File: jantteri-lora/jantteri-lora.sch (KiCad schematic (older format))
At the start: 0 parts

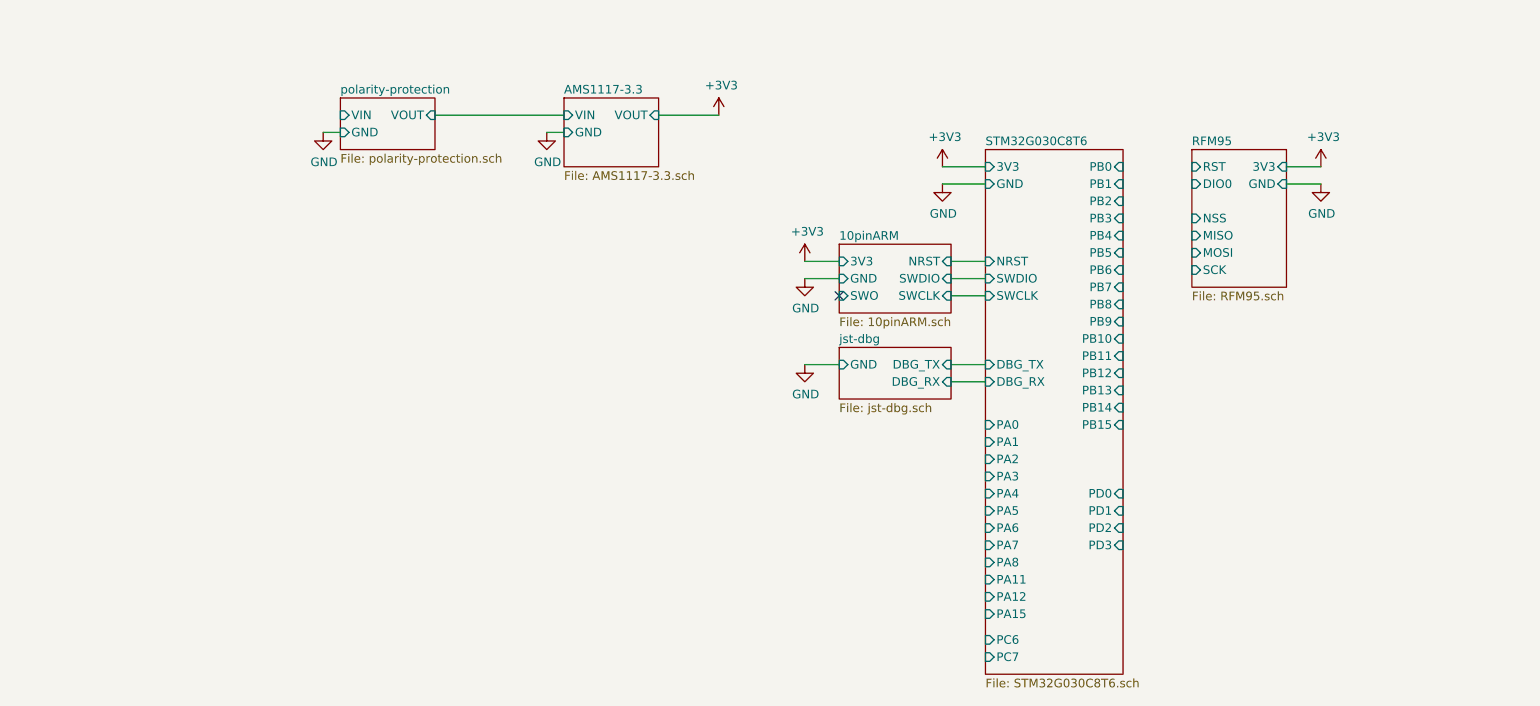
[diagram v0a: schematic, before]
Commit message: Lora PCB desging
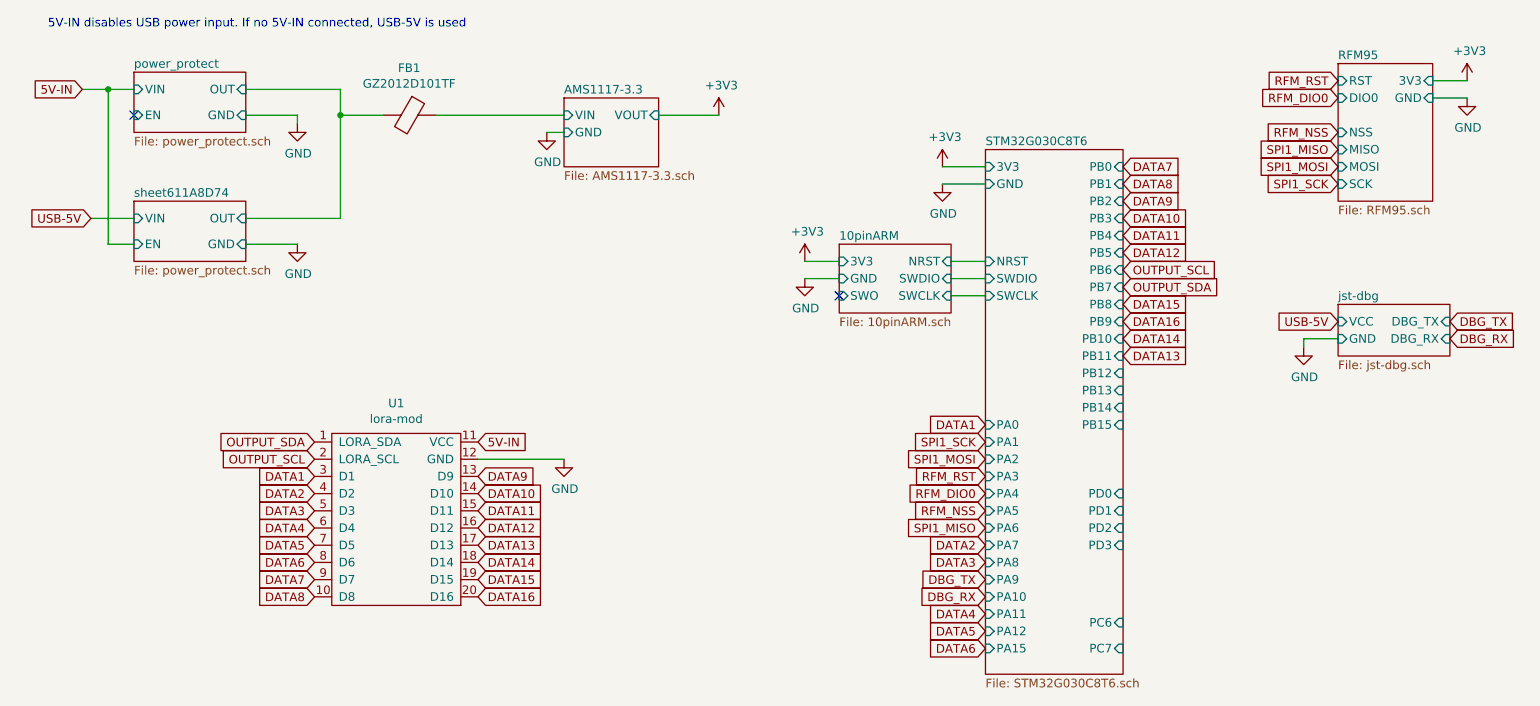
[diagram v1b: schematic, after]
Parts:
- added FB1: GZ2012D101TF, Inductor_SMD:L_0805_2012Metric, symbol Device:Ferrite_Bead
- added U1: lora-mod, RF_Module:HOPERF_RFM69HW, symbol voja-lib:lora-mod
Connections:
- net AMS1117-3.3/VIN: now also FB1.1
- net GND: now also U1.12 (GND)
- new net 5V-IN: U1.11 (VCC)
- new net DATA1: U1.3 (D1)
- new net DATA10: U1.14 (D10)
- new net DATA11: U1.15 (D11)
- new net DATA12: U1.16 (D12)
- new net DATA13: U1.17 (D13)
- new net DATA14: U1.18 (D14)
- new net DATA15: U1.19 (D15)
- new net DATA16: U1.20 (D16)
- new net DATA2: U1.4 (D2)
- new net DATA3: U1.5 (D3)
- new net DATA4: U1.6 (D4)
- new net DATA5: U1.7 (D5)
- new net DATA6: U1.8 (D6)
- new net DATA7: U1.9 (D7)
- new net DATA8: U1.10 (D8)
- new net DATA9: U1.13 (D9)
- new net OUTPUT_SCL: U1.2 (LORA_SCL)
- new net OUTPUT_SDA: U1.1 (LORA_SDA)
- new net power_protect/OUT: FB1.2
- no-connect marks 1 -> 2
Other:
- note added: "5V-IN disables USB power input. If no 5V-IN connected, USB-5V is used"

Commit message: Lora-module v1
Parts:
- U1: footprint RF_Module:HOPERF_RFM69HW -> voja-footprints:lora-mod; symbol voja-lib:lora-mod -> jantteri-lora-rescue:lora-mod-voja-lib
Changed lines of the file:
@@
 $EndSheet
 $Comp
-L power:+3V3 #PWR0101
+L power:+3V3 #PWR08
 U 1 1 61143103
 P 5850 1850
-F 0 "#PWR0101" H 5850 1700 50  0001 C CNN
+F 0 "#PWR08" H 5850 1700 50  0001 C CNN
 F 1 "+3V3" H 5865 2023 50  0000 C CNN
 F 2 "" H 5850 1850 50  0001 C CNN
@@
 $EndComp
 $Comp
-L power:GND #PWR0102
+L power:GND #PWR09
 U 1 1 611435CD
 P 5850 1950
-F 0 "#PWR0102" H 5850 1700 50  0001 C CNN
+F 0 "#PWR09" H 5850 1700 50  0001 C CNN
 F 1 "GND" H 5855 1777 50  0000 C CNN
 F 2 "" H 5850 1950 50  0001 C CNN
@@
 	6100 2600 5900 2600
 $Comp
-L power:GND #PWR0103
+L power:GND #PWR07
 U 1 1 611483EC
 P 5050 2500
-F 0 "#PWR0103" H 5050 2250 50  0001 C CNN
+F 0 "#PWR07" H 5050 2250 50  0001 C CNN
 F 1 "GND" H 5055 2327 50  0000 C CNN
 F 2 "" H 5050 2500 50  0001 C CNN
@@
 $EndComp
 $Comp
-L power:GND #PWR0104
+L power:GND #PWR010
 U 1 1 61148B21
 P 7950 2900
-F 0 "#PWR0104" H 7950 2650 50  0001 C CNN
+F 0 "#PWR010" H 7950 2650 50  0001 C CNN
 F 1 "GND" H 7955 2727 50  0000 C CNN
 F 2 "" H 7950 2900 50  0001 C CNN
@@
 $EndComp
 $Comp
-L power:+3V3 #PWR0105
+L power:+3V3 #PWR06
 U 1 1 61148EAA
 P 5050 2400
-F 0 "#PWR0105" H 5050 2250 50  0001 C CNN
+F 0 "#PWR06" H 5050 2250 50  0001 C CNN
 F 1 "+3V3" H 5065 2573 50  0000 C CNN
 F 2 "" H 5050 2400 50  0001 C CNN
@@
 	5250 2400 5050 2400
 $Comp
-L power:+3V3 #PWR0106
+L power:+3V3 #PWR011
 U 1 1 6114B431
 P 8900 1350
-F 0 "#PWR0106" H 8900 1200 50  0001 C CNN
+F 0 "#PWR011" H 8900 1200 50  0001 C CNN
 F 1 "+3V3" H 8915 1523 50  0000 C CNN
 F 2 "" H 8900 1350 50  0001 C CNN
@@
 $EndComp
 $Comp
-L power:GND #PWR0107
+L power:GND #PWR012
 U 1 1 6114B78E
 P 8900 1450
-F 0 "#PWR0107" H 8900 1200 50  0001 C CNN
+F 0 "#PWR012" H 8900 1200 50  0001 C CNN
 F 1 "GND" H 8905 1277 50  0000 C CNN
 F 2 "" H 8900 1450 50  0001 C CNN
@@
 	8700 1350 8900 1350
 $Comp
-L power:GND #PWR0108
+L power:GND #PWR03
 U 1 1 6114C811
 P 3550 1650
-F 0 "#PWR0108" H 3550 1400 50  0001 C CNN
+F 0 "#PWR03" H 3550 1400 50  0001 C CNN
 F 1 "GND" H 3555 1477 50  0000 C CNN
 F 2 "" H 3550 1650 50  0001 C CNN
@@
 	3550 1650 3650 1650
 $Comp
-L power:+3V3 #PWR0110
+L power:+3V3 #PWR05
 U 1 1 6114D52E
 P 4550 1550
-F 0 "#PWR0110" H 4550 1400 50  0001 C CNN
+F 0 "#PWR05" H 4550 1400 50  0001 C CNN
 F 1 "+3V3" H 4565 1723 50  0000 C CNN
 F 2 "" H 4550 1550 50  0001 C CNN
@@
 5V-IN
 $Comp
-L power:GND #PWR0109
+L power:GND #PWR04
 U 1 1 61169965
 P 3650 3550
-F 0 "#PWR0109" H 3650 3300 50  0001 C CNN
+F 0 "#PWR04" H 3650 3300 50  0001 C CNN
 F 1 "GND" H 3655 3377 50  0000 C CNN
 F 2 "" H 3650 3550 50  0001 C CNN
@@
 DATA1
 $Comp
-L voja-lib:lora-mod U1
+L jantteri-lora-rescue:lora-mod-voja-lib U1
 U 1 1 61170943
 P 2700 3800
 F 0 "U1" H 2675 4375 50  0000 C CNN
 F 1 "lora-mod" H 2675 4284 50  0000 C CNN
-F 2 "RF_Module:HOPERF_RFM69HW" H 2700 3800 50  0001 C CNN
+F 2 "voja-footprints:lora-mod" H 2700 3800 50  0001 C CNN
 F 3 "" H 2700 3800 50  0001 C CNN
 	1    2700 3800
@@
 Connection ~ 2350 1550
 $Comp
-L power:GND #PWR0111
+L power:GND #PWR01
 U 1 1 611AB45E
 P 2100 1600
-F 0 "#PWR0111" H 2100 1350 50  0001 C CNN
+F 0 "#PWR01" H 2100 1350 50  0001 C CNN
 F 1 "GND" H 2105 1427 50  0000 C CNN
 F 2 "" H 2100 1600 50  0001 C CNN
@@
 $EndComp
 $Comp
-L power:GND #PWR0112
+L power:GND #PWR02
 U 1 1 611AB5EF
 P 2100 2300
-F 0 "#PWR0112" H 2100 2050 50  0001 C CNN
+F 0 "#PWR02" H 2100 2050 50  0001 C CNN
 F 1 "GND" H 2105 2127 50  0000 C CNN
 F 2 "" H 2100 2300 50  0001 C CNN
